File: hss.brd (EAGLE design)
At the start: 41.4 x 29 mm, 11 parts, among them IC1 MEGA328P, Q1 BUZ71

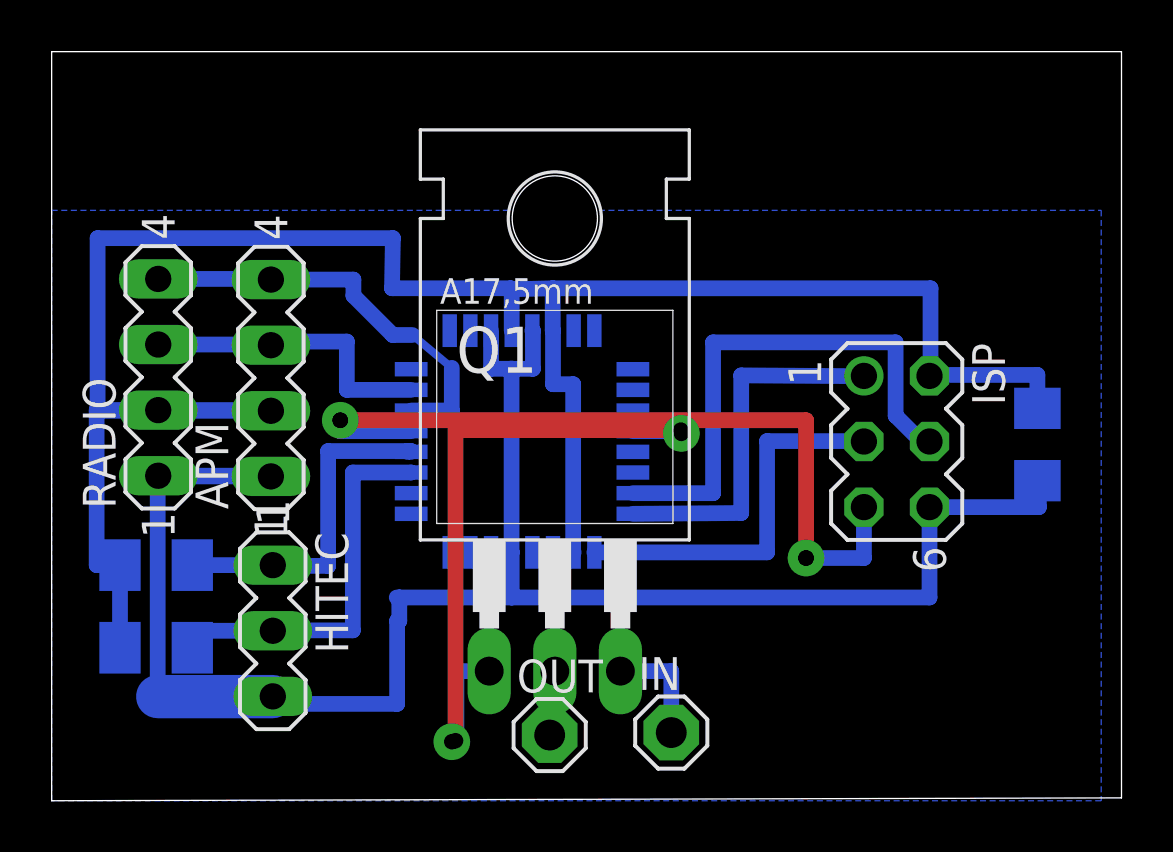
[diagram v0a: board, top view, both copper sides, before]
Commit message: version 4 of the board
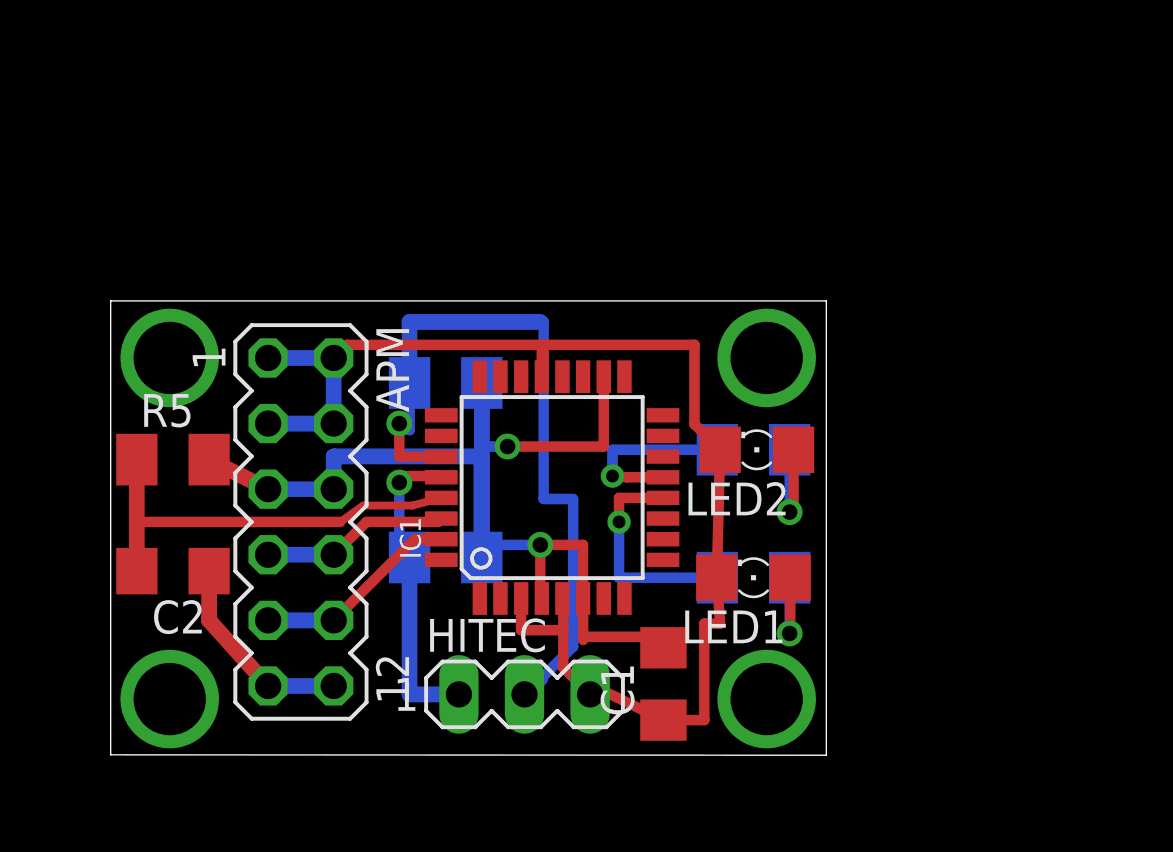
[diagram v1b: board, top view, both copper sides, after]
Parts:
- removed IN, OUT: MCS08, solpad:MCS08
- removed ISP: (no value), con-lstb:MA03-2
- removed Q1: BUZ71, transistor-fet:TO220
- removed RADIO: (no value), con-lstb:MA04-1
- added C2: 100nF, resistor:C1206
- added LED1: GREEN, led:1206
- added LED2: RED, led:1206
- added R3: 68, resistor:M1206
- added R4: 150, resistor:M1206
- added R5: 10k, resistor:M1206
- APM: device con-lstb:MA04-1 -> con-lstb:MA06-2
- moved C1 17.2 mm to (23.7, 4.52), flipped to the top
- moved R1 15.2 mm to (15.3, 16.2), turned to 180 degrees
- moved R2 11.2 mm to (15.3, 9.42), turned to 180 degrees
- moved HITEC 10.1 mm to (18.3, 4.12), turned to 0 degrees
- moved APM 5.69 mm to (9.65, 10.8), turned to 270 degrees
- moved IC1 2.13 mm to (19.4, 12.1), flipped to the top, turned to 90 degrees
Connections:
- removed net N$11: IN.MP, Q1.3
- net GND: now also APM.2, APM.3, APM.4, LED1.C, LED2.C; no longer ISP.6, RADIO.1
- net N$1: now also IC1.12, R3.1; no longer IC1.29, ISP.5
- net N$10: now also APM.11, APM.12, C2.1; no longer IC1.12, Q1.1
- net N$14: now also APM.10, APM.9; no longer APM.3, RADIO.3
- net N$15: now also APM.7, APM.8; no longer APM.4, RADIO.4
- net N$5: now also C2.2, IC1.29, R5.1; no longer OUT.MP, Q1.2
- net N$7: now also LED1.A, R3.2; no longer IC1.17, ISP.3
- net N$8: now also IC1.13, R4.1; no longer IC1.16, ISP.1
- net N$9: now also LED2.A, R4.2; no longer IC1.15, ISP.4
- net VCC: now also APM.5, APM.6, R5.2; no longer APM.2, ISP.2, RADIO.2
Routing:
- net VCC: track 86.1 -> 44.0 mm, vias 0 -> 2
- net GND: track 75.3 -> 51.6 mm
- net N$1: track 30.7 -> 8.60 mm, vias 4 -> 1
- net N$10: track 26.6 -> 7.86 mm, vias 2 -> 0
- net N$9: track 20.6 -> 4.98 mm, vias 0 -> 1
- net N$3: track 15.3 -> 30.0 mm, vias 0 -> 1
- net N$5: track 2.67 -> 16.3 mm
- net N$7: track 14.8 -> 4.35 mm, vias 0 -> 1
- net N$15: track 16.3 -> 7.28 mm
- net N$8: track 14.3 -> 7.03 mm, vias 0 -> 1
- net N$11: track 4.35 -> 0.00 mm, vias 0 -> 3
- net N$14: track 11.8 -> 8.01 mm
- net N$4: track 13.1 -> 12.6 mm, vias 0 -> 1
- removed copper zone on layer 16, net N$13
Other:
- board size 41.4 x 29 mm -> 27.7 x 17.6 mm
- board text added: "APM-HSS"
- board text added: "Adapter"
- board text added: "Janne Mäntyharju"
- board text added: "Rev 4"
